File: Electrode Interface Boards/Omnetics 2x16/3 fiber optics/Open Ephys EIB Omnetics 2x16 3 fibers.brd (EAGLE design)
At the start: 16.1 x 16.1 mm, 40 parts

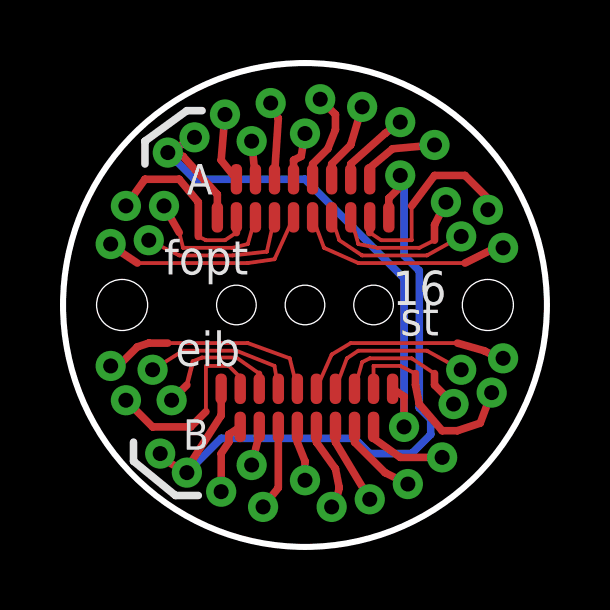
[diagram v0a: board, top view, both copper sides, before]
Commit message: Add Gerber files and images for EIBs
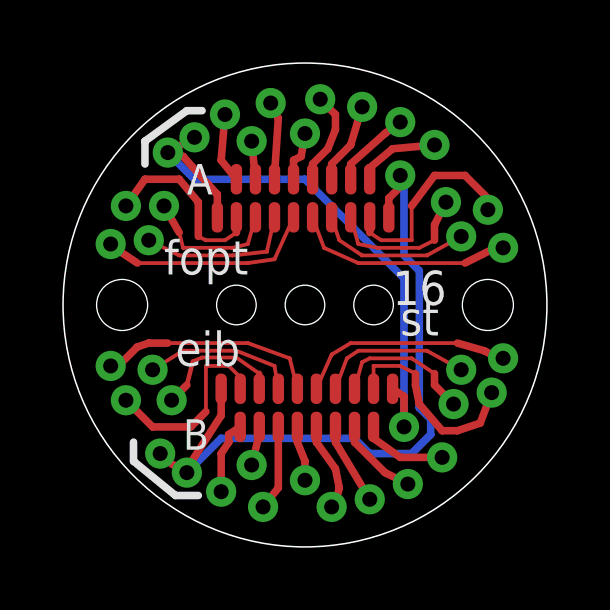
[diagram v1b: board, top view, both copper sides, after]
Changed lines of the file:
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@@
 <?xml version="1.0" encoding="utf-8"?>
 <!DOCTYPE eagle SYSTEM "eagle.dtd">
-<eagle version="6.1">
+<eagle version="6.3">
 <drawing>
 <settings>
@@
 <setting verticaltext="up"/>
 </settings>
-<grid distance="5" unitdist="mil" unit="mil" style="lines" multiple="1" display="yes" altdistance="0.005" altunitdist="inch" altunit="inch"/>
+<grid distance="1" unitdist="mil" unit="mil" style="lines" multiple="1" display="yes" altdistance="0.005" altunitdist="inch" altunit="inch"/>
 <layers>
-<layer number="1" name="Top" color="4" fill="1" visible="yes" active="yes"/>
+<layer number="1" name="Top" color="11" fill="1" visible="yes" active="yes"/>
 <layer number="16" name="Bottom" color="1" fill="1" visible="yes" active="yes"/>
 <layer number="17" name="Pads" color="2" fill="1" visible="yes" active="yes"/>
@@
 <layer number="23" name="tOrigins" color="15" fill="1" visible="yes" active="yes"/>
 <layer number="24" name="bOrigins" color="15" fill="1" visible="yes" active="yes"/>
-<layer number="25" name="tNames" color="7" fill="1" visible="yes" active="yes"/>
+<layer number="25" name="tNames" color="3" fill="1" visible="yes" active="yes"/>
 <layer number="26" name="bNames" color="7" fill="1" visible="yes" active="yes"/>
 <layer number="27" name="tValues" color="7" fill="1" visible="yes" active="yes"/>
@@
 <wire x1="19.685" y1="20.193" x2="21.082" y2="19.05" width="0.254" layer="25"/>
 <wire x1="21.082" y1="19.05" x2="21.844" y2="19.05" width="0.254" layer="25"/>
-<circle x="25.4" y="25.4" radius="8.0645" width="0.2032" layer="20"/>
+<circle x="25.4" y="25.4" radius="8.0645" width="0.0508" layer="20"/>
 <text x="20.701" y="26.416" size="1.143" layer="25" font="vector" ratio="15">fopt</text>
 <text x="21.082" y="23.368" size="1.143" layer="25" font="vector" ratio="15">eib</text>
@@
 </class>
 </classes>
-<designrules>
+<designrules name="default">
 <description language="de">&lt;b&gt;EAGLE Design Rules&lt;/b&gt;
 &lt;p&gt;
